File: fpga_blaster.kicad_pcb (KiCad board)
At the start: 2 copper layers, 193 x 81.9 mm, 238 parts, among them J1 Conn_02x05_Odd_Even, J2 Conn_02x05_Odd_Even, J3 Conn_01x03, J4 Conn_02x05_Odd_Even, J5 HDMI_D_1.4, J8 HDMI_D_1.4, Q1 Pmos, Q2 2N3904, Q4 IPD60R145, Q6 IPD60R145, Q7 2N3906, Q9 2N3904, SW1 FIRE, SW2 SW_DIP_x03, SW3 ARM, U1 LT3420, U10 AMC3330, U11 TLV9102, U12 LTC6362, U13 TLV9102, U14 AMC3302, U15 LTC6362, U16 LTC6362, U17 AD7352, U18 IR2127, U19 S80KS2563GABHV020, U2 MAX10, U20 TLV74318, U21 LM809, U22 MAX3227, U3 AD7352, U4 TLV74325, U5 4945, U6 4945, U7 LTC6362, U8 AMC3330, U9 AMC3302, X1 ASE-48MHz

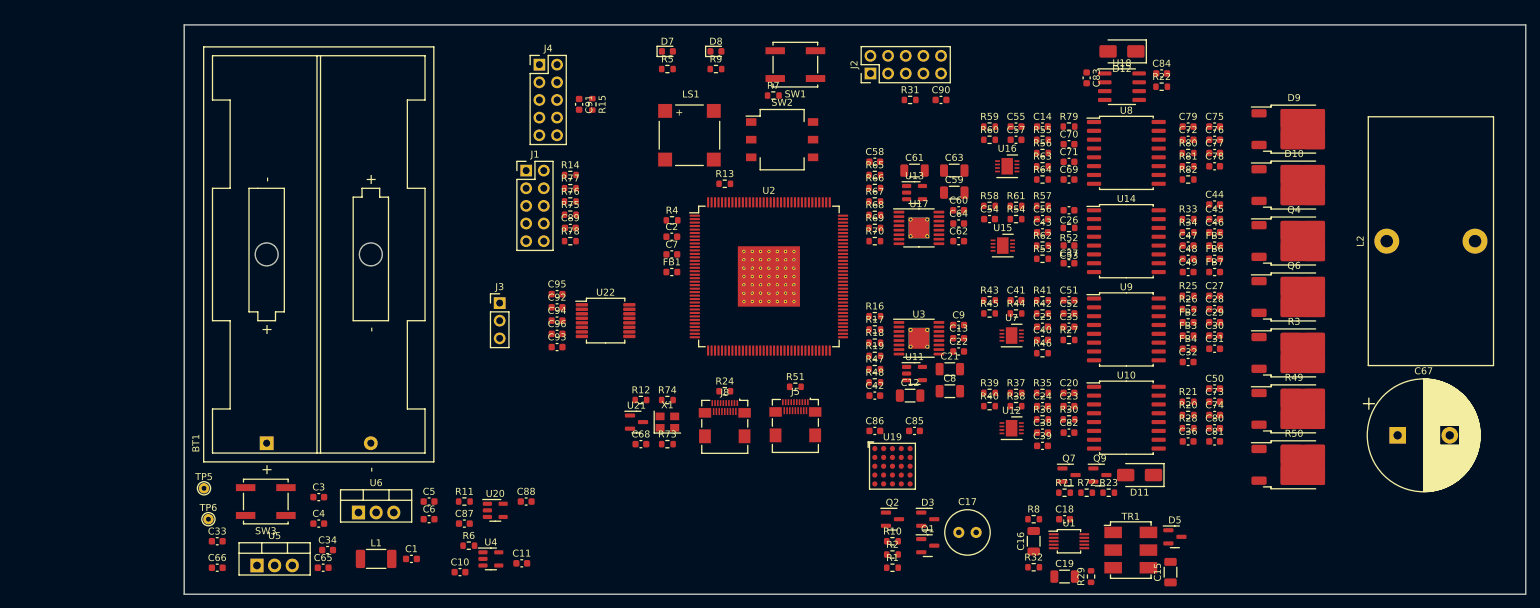
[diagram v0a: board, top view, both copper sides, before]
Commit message: PCB V0.8 tapeout
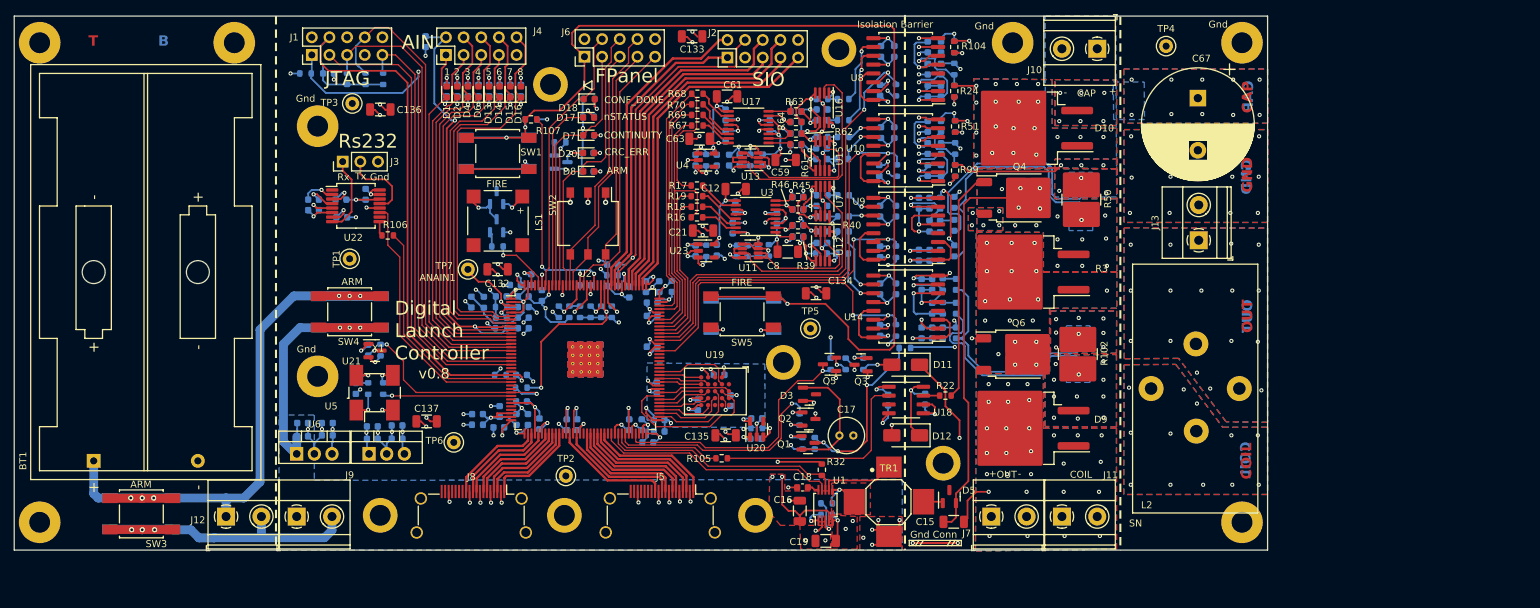
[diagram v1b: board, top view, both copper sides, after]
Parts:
- removed L1: 600uH 0.5A, Inductor_SMD:L_2010_5025Metric
- removed Q9: 2N3904, Package_TO_SOT_SMD:SOT-23
- added ?: , , F.Cu at (223.4, 97.3)
- added ?: , , F.Cu at (223.4, 109.9)
- added C100: 0.1u, Capacitor_SMD:C_0603_1608Metric, B.Cu at (146.1, 108.3)
- added C101: 0.1u, Capacitor_SMD:C_0603_1608Metric, B.Cu at (141.8, 89.9)
- added C102: 0.1u, Capacitor_SMD:C_0603_1608Metric, B.Cu at (134.3, 109.0)
- added C103: 0.1u, Capacitor_SMD:C_0603_1608Metric, B.Cu at (127.3, 108.2)
- added C104: 0.1u, Capacitor_SMD:C_0603_1608Metric, B.Cu at (123.1, 109.3)
- added C105: 0.1u, Capacitor_SMD:C_0603_1608Metric, B.Cu at (123.4, 90.5)
- added C106: 0.1u, Capacitor_SMD:C_0603_1608Metric, B.Cu at (146.1, 89.1)
- added C107: 0.1u, Capacitor_SMD:C_0603_1608Metric, B.Cu at (125.4, 88.9)
- added C108: 0.1u, Capacitor_SMD:C_0603_1608Metric, B.Cu at (126.6, 90.5)
- added C109: 0.1u, Capacitor_SMD:C_0603_1608Metric, B.Cu at (123.2, 107.1)
- added C110: 0.1u, Capacitor_SMD:C_0603_1608Metric, B.Cu at (143.6, 109.0)
- added C111: 0.1u, Capacitor_SMD:C_0603_1608Metric, B.Cu at (127.7, 88.1)
- added C112: 0.1u, Capacitor_SMD:C_0603_1608Metric, B.Cu at (145.1, 91.4)
- added C113: 0.1u, Capacitor_SMD:C_0603_1608Metric, B.Cu at (125.6, 108.2)
- added C114: 0.1u, Capacitor_SMD:C_0603_1608Metric, B.Cu at (126.6, 95.1)
- added C115: 0.1u, Capacitor_SMD:C_0603_1608Metric, B.Cu at (126.3, 101.8)
- added C116: 0.1u, Capacitor_SMD:C_0603_1608Metric, B.Cu at (126.3, 105.6)
- added C117: 0.1u, Capacitor_SMD:C_0603_1608Metric, B.Cu at (132.8, 109.0)
- added C118: 0.1u, Capacitor_SMD:C_0603_1608Metric, B.Cu at (141.8, 109.0)
- added C119: 0.1u, Capacitor_SMD:C_0603_1608Metric, B.Cu at (145.8, 103.6)
- added C120: 0.1u, Capacitor_SMD:C_0603_1608Metric, B.Cu at (139.4, 85.9)
- added C121: 0.1u, Capacitor_SMD:C_0603_1608Metric, B.Cu at (129.3, 90.4)
- added C122: 0.1u, Capacitor_SMD:C_0603_1608Metric, B.Cu at (135.5, 88.9)
- added C123: 0.1u, Capacitor_SMD:C_0603_1608Metric, B.Cu at (145.1, 93.3)
- added C124: 0.1u, Capacitor_SMD:C_0603_1608Metric, B.Cu at (145.1, 97.7)
- added C125: 0.1u, Capacitor_SMD:C_0603_1608Metric, B.Cu at (128.9, 108.8)
- added C126: 0.1u, Capacitor_SMD:C_0603_1608Metric, B.Cu at (156.2, 70.9)
- added C127: 0.1u, Capacitor_SMD:C_0603_1608Metric, B.Cu at (157.4, 84.0)
- added C128: 1u, Capacitor_SMD:C_0603_1608Metric, B.Cu at (151.4, 83.9)
- added C129: 1u, Capacitor_SMD:C_0603_1608Metric, B.Cu at (154.4, 83.8)
- added C130: 1u, Capacitor_SMD:C_0603_1608Metric, B.Cu at (120.0, 107.4)
- added C131: 0.1u, Capacitor_SMD:C_0603_1608Metric, B.Cu at (102.5, 103.7)
- added C132: 4.7u, Capacitor_SMD:C_1206_3216Metric, F.Cu at (122.9, 86.6)
- added C133: 4.7u, Capacitor_SMD:C_1206_3216Metric, F.Cu at (150.9, 53.1)
- added C134: 4.7u, Capacitor_SMD:C_1206_3216Metric, F.Cu at (168.7, 90.1)
- added C135: 4.7u, Capacitor_SMD:C_1206_3216Metric, F.Cu at (155.7, 110.5)
- added C136: 4.7u, Capacitor_SMD:C_1206_3216Metric, F.Cu at (106.0, 63.6)
- added C137: 4.7u, Capacitor_SMD:C_1206_3216Metric, F.Cu at (112.7, 108.5)
- added C97: 0.1u, Capacitor_SMD:C_0603_1608Metric, B.Cu at (154.7, 101.8)
- added C98: 0.1u, Capacitor_SMD:C_0603_1608Metric, B.Cu at (144.2, 89.1)
- added C99: 0.1u, Capacitor_SMD:C_0603_1608Metric, B.Cu at (146.1, 109.9)
- added D1: Yel, LED_SMD:LED_0603_1608Metric, F.Cu at (117.1, 61.1)
- added D13: Yel, LED_SMD:LED_0603_1608Metric, F.Cu at (121.7, 61.1)
- added D14: Yel, LED_SMD:LED_0603_1608Metric, F.Cu at (123.2, 61.1)
- added D15: Yel, LED_SMD:LED_0603_1608Metric, F.Cu at (124.7, 61.1)
- added D16: Yel, LED_SMD:LED_0603_1608Metric, F.Cu at (126.2, 61.1)
- added D17: nSTATUS, LED_SMD:LED_0603_1608Metric, F.Cu at (136.0, 64.8)
- added D18: CONF_DONE, LED_SMD:LED_0603_1608Metric, F.Cu at (136.1, 62.1)
- added D19: BAV99, Package_TO_SOT_SMD:SOT-23, B.Cu at (122.7, 76.3)
- added D2: Yel, LED_SMD:LED_0603_1608Metric, F.Cu at (115.6, 61.1)
- added D20: CRC_ERR, LED_SMD:LED_0603_1608Metric, F.Cu at (136.0, 69.8)
- added D4: Yel, LED_SMD:LED_0603_1608Metric, F.Cu at (118.6, 61.1)
- added D6: Yel, LED_SMD:LED_0603_1608Metric, F.Cu at (120.1, 61.1)
- added FB10: Ferrite, Inductor_SMD:L_0603_1608Metric, B.Cu at (120.0, 109.0)
- added FB11: Ferrite, Inductor_SMD:L_0603_1608Metric, B.Cu at (144.5, 111.5)
- added FB8: Ferrite, Inductor_SMD:L_0603_1608Metric, B.Cu at (148.0, 89.1)
- added FB9: Ferrite, Inductor_SMD:L_0603_1608Metric, B.Cu at (120.9, 91.3)
- added H1: ~, MountingHole:MountingHole_3mm_Pad, F.Cu at (57.0, 54.0)
- added H10: ~, MountingHole:MountingHole_3mm_Pad, F.Cu at (57.0, 123.0)
- added H11: ~, MountingHole:MountingHole_3mm_Pad, F.Cu at (130.5, 60.0)
- added H12: ~, MountingHole:MountingHole_3mm_Pad, F.Cu at (230.0, 123.0)
- added H13: ~, MountingHole:MountingHole_3mm_Pad, F.Cu at (160.0, 122.0)
- added H14: ~, MountingHole:MountingHole_3mm_Pad, F.Cu at (106.0, 122.0)
- added H15: ~, MountingHole:MountingHole_3mm_Pad, F.Cu at (187.0, 114.5)
- added H2: ~, MountingHole:MountingHole_3mm_Pad, F.Cu at (85.0, 54.0)
- added H3: ~, MountingHole:MountingHole_3mm_Pad, F.Cu at (172.0, 55.0)
- added H4: ~, MountingHole:MountingHole_3mm_Pad, F.Cu at (197.0, 54.0)
- added H5: ~, MountingHole:MountingHole_3mm_Pad, F.Cu at (230.0, 54.0)
- added H6: ~, MountingHole:MountingHole_3mm_Pad, F.Cu at (97.0, 66.0)
- added H7: ~, MountingHole:MountingHole_3mm_Pad, F.Cu at (97.0, 102.0)
- added H8: ~, MountingHole:MountingHole_3mm_Pad, F.Cu at (164.0, 100.0)
- added H9: ~, MountingHole:MountingHole_3mm_Pad, F.Cu at (132.5, 122.0)
- added J10: Screw_Terminal_01x02, TerminalBlock_Phoenix:TerminalBlock_Phoenix_MKDS-1,5-2-5.08_1x02_P5.08mm_Horizontal, F.Cu at (209.2, 54.9)
- added J11: Screw_Terminal_01x02, TerminalBlock_Phoenix:TerminalBlock_Phoenix_MKDS-1,5-2-5.08_1x02_P5.08mm_Horizontal, F.Cu at (204.1, 122.2)
- added J12: Screw_Terminal_01x02, TerminalBlock_Phoenix:TerminalBlock_Phoenix_MKDS-1,5-2-5.08_1x02_P5.08mm_Horizontal, F.Cu at (83.8, 122.2)
- added J13: Screw_Terminal_01x02, TerminalBlock_Phoenix:TerminalBlock_Phoenix_MKDS-1,5-2-5.08_1x02_P5.08mm_Horizontal, F.Cu at (223.8, 82.4)
- added J6: Conn_02x05_Odd_Even, Connector_PinHeader_2.54mm:PinHeader_2x05_P2.54mm_Vertical, F.Cu at (135.4, 56.0)
- added J7: Screw_Terminal_01x02, TerminalBlock_Phoenix:TerminalBlock_Phoenix_MKDS-1,5-2-5.08_1x02_P5.08mm_Horizontal, F.Cu at (193.9, 122.2)
- added J9: Screw_Terminal_01x02, TerminalBlock_Phoenix:TerminalBlock_Phoenix_MKDS-1,5-2-5.08_1x02_P5.08mm_Horizontal, F.Cu at (94.0, 122.2)
- added Q3: 2N3906, Package_TO_SOT_SMD:SOT-23, F.Cu at (175.2, 100.3)
- added Q5: 2N3904, Package_TO_SOT_SMD:SOT-23, F.Cu at (170.6, 100.3)
- added Q8: 2N3904, Package_TO_SOT_SMD:SOT-23, B.Cu at (132.0, 71.2)
- added R100: 0R, Resistor_SMD:R_0603_1608Metric, B.Cu at (206.9, 78.7)
- added R101: 0R, Resistor_SMD:R_0603_1608Metric, B.Cu at (206.9, 74.4)
- added R102: 0.005R 1W, myspace pcb:R_2818 current sense, F.Cu at (206.4, 98.8)
- added R103: 0R, Resistor_SMD:R_0603_1608Metric, B.Cu at (206.5, 96.8)
- added R104: 0R, Resistor_SMD:R_0603_1608Metric, F.Cu at (188.6, 54.6)
- added R105: 22R, Resistor_SMD:R_0603_1608Metric, F.Cu at (155.1, 113.8)
- added R106: 22R, Resistor_SMD:R_0603_1608Metric, F.Cu at (107.1, 81.7)
- added R107: 22R, Resistor_SMD:R_0603_1608Metric, F.Cu at (127.7, 65.0)
- added R108: 1K, Resistor_SMD:R_0603_1608Metric, B.Cu at (122.9, 83.3)
- added R109: 1K, Resistor_SMD:R_0603_1608Metric, B.Cu at (135.8, 69.8)
- added R110: 0R, Resistor_SMD:R_0603_1608Metric, B.Cu at (181.5, 97.9)
- added R111: 1K, Resistor_SMD:R_0603_1608Metric, B.Cu at (131.9, 68.3)
- added R112: DNI, Resistor_SMD:R_0603_1608Metric, B.Cu at (126.3, 103.6)
- added R83: 1K, Resistor_SMD:R_0603_1608Metric, B.Cu at (117.1, 60.8)
- added R84: 1K, Resistor_SMD:R_0603_1608Metric, B.Cu at (115.6, 60.8)
- added R85: 1K, Resistor_SMD:R_0603_1608Metric, B.Cu at (118.6, 60.8)
- added R86: 1K, Resistor_SMD:R_0603_1608Metric, B.Cu at (120.1, 60.8)
- added R87: 1K, Resistor_SMD:R_0603_1608Metric, B.Cu at (121.7, 60.8)
- added R88: 1K, Resistor_SMD:R_0603_1608Metric, B.Cu at (123.2, 60.8)
- added R89: 1K, Resistor_SMD:R_0603_1608Metric, B.Cu at (124.7, 60.8)
- added R90: 1K, Resistor_SMD:R_0603_1608Metric, B.Cu at (126.2, 60.8)
- added R91: 1K, Resistor_SMD:R_0603_1608Metric, B.Cu at (136.0, 64.6)
- added R92: 1K, Resistor_SMD:R_0603_1608Metric, B.Cu at (136.0, 62.1)
- added R93: DNI, Resistor_SMD:R_0603_1608Metric, B.Cu at (133.2, 92.7)
- added R94: DNI, Resistor_SMD:R_0603_1608Metric, B.Cu at (134.7, 92.7)
- added R95: 10K, Resistor_SMD:R_0603_1608Metric, B.Cu at (131.7, 92.7)
- added R96: DNI, Resistor_SMD:R_0603_1608Metric, B.Cu at (137.8, 92.7)
- added R97: DNI, Resistor_SMD:R_0603_1608Metric, B.Cu at (136.3, 92.7)
- added R98: 10K, Resistor_SMD:R_0603_1608Metric, B.Cu at (152.9, 83.9)
- added R99: 0R, Resistor_SMD:R_0603_1608Metric, F.Cu at (188.7, 72.4)
- added SW4: ARM, myspace pcb:SW_SPST_HP03, F.Cu at (101.6, 92.7)
- added SW5: FIRE, myspace pcb:SW_SPST_HP03, F.Cu at (158.1, 92.7)
- added SW6: FIRE, myspace pcb:SW_SPST_HP03, B.Cu at (158.1, 93.1)
- added SW7: ARM, myspace pcb:SW_SPST_HP03, B.Cu at (101.7, 92.7)
- added SW8: ARM, myspace pcb:SW_SPST_HP03, B.Cu at (71.6, 121.8)
- added SW9: FIRE, myspace pcb:SW_SPST_HP03, B.Cu at (122.9, 69.9)
- added TP1: ~, TestPoint:TestPoint_Keystone_5000-5004_Miniature, F.Cu at (101.6, 85.1)
- added TP2: ~, TestPoint:TestPoint_Keystone_5000-5004_Miniature, F.Cu at (132.7, 116.3)
- added TP3: ~, TestPoint:TestPoint_Keystone_5000-5004_Miniature, F.Cu at (102.0, 62.7)
- added TP4: ~, TestPoint:TestPoint_Keystone_5000-5004_Miniature, F.Cu at (219.1, 54.5)
- added TP7: ~, TestPoint:TestPoint_Keystone_5000-5004_Miniature, F.Cu at (118.6, 86.6)
- added U23: TLV74325, Package_TO_SOT_SMD:SOT-23-5, F.Cu at (152.9, 83.9)
- BT1: value 2xAA Li -> ~
- C1, C10, C11, C13, C14, C20, C22, C24, C25, C26, C3, C30, C33, C34, C4, C42, C43, C45, C5, C50, C51, C58, C6, C60, C62, C64, C65, C66, C68, C7, C70, C75, C83, C84, C87, C88, C89, C9, C90, C91, C92, C93, C94, C95, C96, FB1, FB2, FB3, FB4, FB5, FB6, FB7, R1, R10, R11, R13, R14, R15, R2, R20, R21, R23, R25, R26, R27, R28, R29, R30, R31, R33, R34, R35, R36, R37, R38, R4, R41, R42, R43, R44, R5, R52, R53, R54, R55, R56, R57, R58, R59, R6, R60, R7, R71, R72, R73, R75, R76, R77, R78, R79, R8, R80, R81, R82, R9: moved to B.Cu
- C17: footprint Capacitor_THT:C_Radial_D6.3mm_H5.0mm_P2.50mm -> Capacitor_THT:C_Radial_D5.0mm_H7.0mm_P2.00mm
- C2: value 0.1u -> 0.001u; moved to B.Cu
- C23, C28, C31, C37, C38, C39, C40, C41, C47, C48, C52, C54, C55, C56, C57, C71, C74, C77, C78, C80: value 1n -> 0.001u; moved to B.Cu
- C27, C36, C44, C72: value 10n -> 0.01u; moved to B.Cu
- C29, C32, C35, C46, C49, C53, C69, C73, C76, C79, C81, C82: value 100n -> 0.1u; moved to B.Cu
- C85: value 1u -> 0.1u; moved to B.Cu
- C86: value 1n -> 0.1u; moved to B.Cu
- D10, D9, R3: footprint Package_TO_SOT_SMD:TO-252-2 -> Package_TO_SOT_SMD:TO-263-2_TabPin1
- D11, D12: value SBYV26C -> ES1J
- D3: value 1N4001 -> BAV99
- D5: value MMBD3004SE -> GSD2004S
- D7: value FIRE -> CONTINUITY
- J5, J8: footprint Connector_HDMI:HDMI_Micro-D_Molex_46765-0x01 -> Connector_HDMI:HDMI_A_Amphenol_10029449-x01xLF_Horizontal
- Q1: value Pmos -> STR2P3LLH6(Pfet)
- Q7: value 2N3906 -> 2N3904; moved to B.Cu
- R12, R74: value 1K -> 22R; moved to B.Cu
- R22: value 2R -> 10R
- R39, R40, R45, R46, R61, R62, R63, R64: value 30R -> 22R
- R47, R48, R65, R66: value 10.0K -> 10.01K; moved to B.Cu
- R49: value 0.005R 1W -> 0R; footprint Package_TO_SOT_SMD:TO-252-2 -> Resistor_SMD:R_0603_1608Metric; moved to B.Cu
- R50: footprint Package_TO_SOT_SMD:TO-252-2 -> myspace pcb:R_2818 current sense
- SW1, SW3: footprint Button_Switch_SMD:SW_Push_1P1T_NO_CK_KSC6xxJ -> myspace pcb:SW_SPST_HP03
- TP5: value 3V -> ~; footprint TestPoint:TestPoint_THTPad_D1.5mm_Drill0.7mm -> TestPoint:TestPoint_Keystone_5000-5004_Miniature
- TP6: value GND -> ~; footprint TestPoint:TestPoint_THTPad_D1.5mm_Drill0.7mm -> TestPoint:TestPoint_Keystone_5000-5004_Miniature
- TR1: footprint RF_Mini-Circuits:Mini-Circuits_CD542_H2.84mm -> myspace pcb:PA0637A Pulse Coil
- U11, U13: value TLV9102 -> TLV9062xD; footprint Package_TO_SOT_SMD:SOT-23-5 -> Package_TO_SOT_SMD:SOT-23-8
- U12, U15, U16, U7: footprint Package_DFN_QFN:DFN-8-1EP_3x3mm_P0.5mm_EP1.66x2.38mm -> Package_SO:MSOP-8_3x3mm_P0.65mm
- U17, U3: footprint Package_SO:TSSOP-16-1EP_4.4x5mm_P0.65mm_EP3x3mm_ThermalVias -> Package_SO:TSSOP-16_4.4x5mm_P0.65mm
- U19: footprint Package_BGA:BGA-25_6.35x6.35mm_Layout5x5_P1.27mm -> myspace pcb:FBGA-24_6mmx8mm_Layout5x5_P1.00mm
- U2: value MAX10 -> MAX10M04; footprint Package_QFP:EQFP-144-1EP_20x20mm_P0.5mm_EP8.93x8.7mm_ThermalVias -> Package_QFP:EQFP-144-1EP_20x20mm_P0.5mm_EP5x5mm_ThermalVias
- U5: value 4945 -> LMO78_03-1.0
- X1: footprint Oscillator:Oscillator_SMD_Abracon_ASE-4Pin_3.2x2.5mm -> Oscillator:Oscillator_SMD_Abracon_ASV-4Pin_7.0x5.1mm_HandSoldering
- moved TP5 90.2 mm to (167.9, 95.1)
- moved Q7 89.8 mm to (122.7, 80.3), turned to 90 degrees
- moved C10 68.3 mm to (151.4, 70.9), turned to -90 degrees
- moved U4 65.2 mm to (152.9, 70.9)
- moved R6 65.1 mm to (152.9, 70.9), turned to -90 degrees
- moved C11 64.4 mm to (154.4, 70.9), turned to -90 degrees
- moved D12 63.4 mm to (181.6, 110.5)
- moved C81 59.0 mm to (184.8, 69.2), turned to -90 degrees
- moved C74 58.5 mm to (184.8, 66.0), turned to -90 degrees
- moved D9 58.3 mm to (198.1, 109.5), turned to 180 degrees
- moved C84 57.9 mm to (184.4, 105.3), turned to -90 degrees
- moved C36 57.6 mm to (186.7, 66.0), turned to 90 degrees
- moved C67 56.4 mm to (223.6, 62.0), turned to -90 degrees
- moved C80 55.5 mm to (184.8, 72.4), turned to 90 degrees
- moved U18 54.7 mm to (181.7, 105.4)
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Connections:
- net Net-(BT1-+) renamed /B+
- net Net-(J1-Pin_4) renamed /VCCIO1B
- net Net-(J4-Pin_2) renamed /VCCIO1A
- net Net-(Q6-D) renamed /SWDIS
- net Net-(U1-SW) renamed /SW
- net Net-(U10-DCDC_HGND) renamed /HGNDCV
- net Net-(U14-DCDC_HGND) renamed /HGNDLI
- net Net-(U2A-ANAIN1) renamed /ANAIN1
- net Net-(U8-DCDC_HGND) renamed /HGNDLV
- net Net-(U8-OUTN) renamed /LVoutn
- net Net-(U8-OUTP) renamed /LVoutp
- net Net-(U9-DCDC_HGND) renamed /HGNDCI
- net Net-(U9-OUTN) renamed /CIoutn
- net Net-(U9-OUTP) renamed /CIoutp
- BT1 pad 2: CVlo -> GND
- C1 pad 2: CVlo -> GND
- C10 pad 2: CVlo -> GND
- C11 pad 2: CVlo -> GND
- C12 pad 2: CVlo -> GND
- C13 pad 2: CVlo -> GND
- C14 pad 1: +2V5 -> +3.3V
- C14 pad 2: CVlo -> GND
- C15 pad 1: CIlo -> +300V
- C15 pad 2: CVlo -> GND
- C16 pad 2: CVlo -> GND
- C17 pad 2: CVlo -> GND
- C18 pad 2: CVlo -> GND
- C19 pad 2: CVlo -> GND
- C2 pad 2: CVlo -> /REFGND
- C20 pad 2: CVlo -> GND
- C21 pad 2: CVlo -> GND
- C22 pad 2: CVlo -> GND
- C23 pad 2: CVlo -> GND
- C24 pad 1: +2V5 -> +3.3V
- C24 pad 2: CVlo -> GND
- C25 pad 1: +2V5 -> +3.3V
- C25 pad 2: CVlo -> GND
- C26 pad 2: CVlo -> GND
- C3 pad 2: CVlo -> GND
- C33 pad 2: CVlo -> GND
- C34 pad 2: CVlo -> GND
- C37 pad 2: CVlo -> GND
- C38 pad 1: /vinb0+ -> /vina0+
- C38 pad 2: CVlo -> GND
- C39 pad 1: /vinb0- -> /vina0-
- C39 pad 2: CVlo -> GND
- C4 pad 2: CVlo -> GND
- C40 pad 1: /vina0+ -> /vinb0+
- C40 pad 2: CVlo -> GND
- C41 pad 1: /vina0- -> /vinb0-
- C41 pad 2: CVlo -> GND
- C42 pad 2: CVlo -> GND
- C43 pad 1: +2V5 -> +3.3V
- C43 pad 2: CVlo -> GND
- C5 pad 2: CVlo -> GND
- C51 pad 2: CVlo -> GND
- C52 pad 2: CVlo -> GND
- C54 pad 2: CVlo -> GND
- C55 pad 2: CVlo -> GND
- C56 pad 2: CVlo -> GND
- C57 pad 2: CVlo -> GND
- C58 pad 2: CVlo -> GND
- C59 pad 2: CVlo -> GND
- C6 pad 2: CVlo -> GND
- C60 pad 2: CVlo -> GND
- C61 pad 2: CVlo -> GND
- C62 pad 2: CVlo -> GND
- C63 pad 2: CVlo -> GND
- C64 pad 2: CVlo -> GND
- C65 pad 2: CVlo -> GND
- C66 pad 2: CVlo -> GND
- C67 pad 1: CIhi -> /CSEN
- C67 pad 2: CVlo -> GND
- C68 pad 2: CVlo -> GND
- C7 pad 2: CVlo -> GND
- C70 pad 2: CVlo -> GND
- C71 pad 2: CVlo -> GND
- C8 pad 2: CVlo -> GND
- C83 pad 2: CVlo -> GND
- C84 pad 2: Net-(D9-K) -> +VSW
- C85 pad 2: CVlo -> GND
- C86 pad 2: CVlo -> GND
- C87 pad 2: CVlo -> GND
- C88 pad 2: CVlo -> GND
- C89 pad 2: CVlo -> GND
- C9 pad 2: CVlo -> GND
- C90 pad 1: Net-(J2-Pin_10) -> /vccio7
- C90 pad 2: CVlo -> GND
- C91 pad 2: CVlo -> GND
- C93 pad 2: CVlo -> GND
- C95 pad 2: CVlo -> GND
- C96 pad 2: CVlo -> GND
- D10 pad 1: LIhi -> /+OUT
- D10 pad 2: CIlo -> +300V
- D11 pad 1: IGNITER+ -> /+OUT
- D5 pad 2: CIlo -> +300V
- D9 pad 1: CVlo -> GND
- D9 pad 2: Net-(D9-K) -> +VSW
- FB1 pad 1: Net-(U2A-REFGDN) -> /REFGND
- FB1 pad 2: CVlo -> GND
- FB6 pad 2: IGNITER+ -> LIlo
- FB7 pad 2: IGNITER+ -> LIlo
- J1 pad 10: CVlo -> GND
- J1 pad 2: CVlo -> GND
- J2 pad 1: Net-(J2-Pin_1) -> /dio0
- J2 pad 10: Net-(J2-Pin_10) -> GND
- J2 pad 2: Net-(J2-Pin_2) -> /dio1
- J2 pad 3: Net-(J2-Pin_3) -> GND
- J2 pad 4: CVlo -> /vccio7
- J2 pad 5: CVlo -> /dio2
- J2 pad 6: Net-(J2-Pin_6) -> /dio3
- J2 pad 7: Net-(J2-Pin_7) -> /dio4
- J2 pad 8: Net-(J2-Pin_8) -> /dio5
- J2 pad 9: Net-(J2-Pin_9) -> /dio6
- J3 pad 1: /tx232 -> /rx232
- J3 pad 2: /rx232 -> /tx232
- J3 pad 3: CVlo -> GND
- J4 pad 4: /ain_5 -> /ain_3
- J4 pad 5: /ain_3 -> /ain_4
- J4 pad 6: /ain_6 -> /ain_5
- J4 pad 7: /ain_4 -> /ain_6
- J4 pad 9: CVlo -> GND
- J5 pad 1: unconnected-(J5-HPD/HEAC--Pad1) -> /hdmi2_d2+
- J5 pad 10: unconnected-(J5-D0S-Pad10) -> /hdmi2_ck+
- J5 pad 11: /hdmi_d0- -> GND
- J5 pad 12: /hdmi_ck+ -> /hdmi2_ck-
- J5 pad 14: /hdmi_ck- -> unconnected-(J5-UTILITY-Pad14)
- J5 pad 16: CVlo -> unconnected-(J5-SDA-Pad16)
- J5 pad 17: unconnected-(J5-SCL-Pad17) -> GND
- J5 pad 2: unconnected-(J5-UTILITY/HEAC+-Pad2) -> GND
- J5 pad 3: /hdmi_d2+ -> /hdmi2_d2-
- J5 pad 4: unconnected-(J5-D2S-Pad4) -> /hdmi2_d1+
- J5 pad 5: /hdmi_d2- -> GND
- J5 pad 6: /hdmi_d1+ -> /hdmi2_d1-
- J5 pad 7: unconnected-(J5-D1S-Pad7) -> /hdmi2_d0+
- J5 pad 8: /hdmi_d1- -> GND
- J5 pad 9: /hdmi_d0+ -> /hdmi2_d0-
- J5 pad SH: Net-(J5-PadSH) -> GND
- J8 pad 1: unconnected-(J8-HPD/HEAC--Pad1) -> /hdmi_d2+
- J8 pad 10: unconnected-(J8-D0S-Pad10) -> /hdmi_ck+
- J8 pad 11: /hdmi_d0- -> GND
- J8 pad 12: /hdmi_ck+ -> /hdmi_ck-
- J8 pad 14: /hdmi_ck- -> unconnected-(J8-UTILITY-Pad14)
- J8 pad 16: CVlo -> unconnected-(J8-SDA-Pad16)
- J8 pad 17: unconnected-(J8-SCL-Pad17) -> GND
- J8 pad 2: unconnected-(J8-UTILITY/HEAC+-Pad2) -> GND
- J8 pad 3: /hdmi_d2+ -> /hdmi_d2-
- J8 pad 4: unconnected-(J8-D2S-Pad4) -> /hdmi_d1+
- J8 pad 5: /hdmi_d2- -> GND
- J8 pad 6: /hdmi_d1+ -> /hdmi_d1-
- J8 pad 7: unconnected-(J8-D1S-Pad7) -> /hdmi_d0+
- J8 pad 8: /hdmi_d1- -> GND
- J8 pad 9: /hdmi_d0+ -> /hdmi_d0-
- J8 pad SH: Net-(J8-PadSH) -> GND
- L2 pad 1: Net-(D9-K) -> /LSEN
- L2 pad 2: LIhi -> /+OUT
- LS1 pad 1: /spk+ -> +3.3V
- LS1 pad 2: /spk- -> Net-(D19-A)
- Q2 pad 1: CVlo -> GND
- Q4 pad 1: Net-(Q4-G) -> /gate
- Q4 pad 2: CIlo -> +300V
- Q4 pad 3: Net-(D9-K) -> +VSW
- Q6 pad 1: Net-(Q1-D) -> /DisG
- Q6 pad 3: CVlo -> GND
- Q7 pad 1: +12V -> GND
- Q7 pad 3: Net-(Q7-C) -> Net-(D19-A)
- R1 pad 1: CVlo -> GND
- R18 pad 1: /dataa0 -> /dataA0
- R19 pad 1: /datab0 -> /dataB0
- R2 pad 1: CVlo -> GND
- R20 pad 1: CIhi -> CVhi
- R22 pad 1: /gate -> Net-(U18-HO)
- R22 pad 2: Net-(Q4-G) -> /gate
- R23 pad 1: Net-(Q7-B) -> Net-(Q3-B)
- R24 pad 1: Net-(J8-PadSH) -> LVhi
- R24 pad 2: CVlo -> /+OUT
- R3 pad 2: CIlo -> +300V
- R31 pad 2: Net-(J2-Pin_10) -> /vccio7
- R35 pad 1: Net-(U10-OUTN) -> /LIoutn
- R36 pad 1: Net-(U10-OUTP) -> /LIoutp
- R39 pad 2: /vinb0+ -> /vina0+
- R4 pad 2: CVlo -> GND
- R40 pad 2: /vinb0- -> /vina0-
- R45 pad 2: /vina0+ -> /vinb0+
- R46 pad 2: /vina0- -> /vinb0-
- R48 pad 1: CVlo -> GND
- R49 pad 1: IGNITER+ -> +VSW
- R50 pad 1: CIhi -> /CSEN
- R50 pad 2: CIlo -> +300V
- R51 pad 1: Net-(J5-PadSH) -> CVlo
- R51 pad 2: CVlo -> GND
- R53 pad 1: Net-(U14-OUTP) -> /CVoutp
- R54 pad 1: Net-(U14-OUTN) -> /CVoutn
- R66 pad 1: CVlo -> GND
- R69 pad 1: /dataa1 -> /dataA1
- R7 pad 2: CVlo -> GND
- R70 pad 1: /datab1 -> /dataB1
- R71 pad 2: Net-(Q7-C) -> Net-(Q3-C)
- R77 pad 2: /tdi -> /tms
- R78 pad 2: CVlo -> GND
- R8 pad 2: CVlo -> GND
- R80 pad 1: IGNITER+ -> LVhi
- R81 pad 1: CVlo -> LVlo
- SW2 pad 1: CVlo -> GND
- SW2 pad 2: CVlo -> GND
- SW2 pad 3: CVlo -> GND
- TP5 pad 1: +BATT -> GND
- TP6 pad 1: CVlo -> GND
- U1 pad 5: CVlo -> GND
- U10 pad 10: Net-(U10-OUTN) -> /CVoutn
- U10 pad 11: Net-(U10-OUTP) -> /CVoutp
- U10 pad 9: CVlo -> GND
- U11 pad 4: (no net) -> GND
- U11 pad 5: (no net) -> Net-(U11A-+)
- U12 pad 3: +2V5 -> +3.3V
- U12 pad 6: CVlo -> GND
- U12 pad 7: +2V5 -> +3.3V
- U13 pad 4: (no net) -> GND
- U13 pad 5: (no net) -> Net-(U13A-+)
- U14 pad 10: Net-(U14-OUTN) -> /LIoutn
- U14 pad 11: Net-(U14-OUTP) -> /LIoutp
- U14 pad 9: CVlo -> GND
- U15 pad 3: +2V5 -> +3.3V
- U15 pad 6: CVlo -> GND
- U15 pad 7: +2V5 -> +3.3V
- U16 pad 2: Net-(U13A--) -> Net-(U13B--)
- U16 pad 3: +2V5 -> +3.3V
- U16 pad 6: CVlo -> GND
- U16 pad 7: +2V5 -> +3.3V
- U17 pad 11: CVlo -> GND
- U17 pad 12: CVlo -> GND
- U17 pad 4: CVlo -> GND
- U17 pad 5: CVlo -> GND
- U18 pad 2: /pwm -> /pwmr
- U18 pad 4: CVlo -> GND
- U18 pad 5: Net-(D9-K) -> +VSW
- U18 pad 6: Net-(D9-K) -> +VSW
- U18 pad 7: /gate -> Net-(U18-HO)
- U19 pad A4: (no net) -> /spi_nrst
- U19 pad B1: unconnected-(U19-nCK-PadB1) -> +1V8
- U19 pad B3: CVlo -> GND
- U19 pad C1: CVlo -> GND
- U19 pad E5: CVlo -> GND
- U2 pad 10: /ain_4 -> /ain_5
- U2 pad 100: unconnected-(U2H-IO-Pad100) -> /dataB0
- U2 pad 101: /LIdiag -> /sclk
- U2 pad 102: /LVdiag -> /dataA1
- U2 pad 104: CVlo -> GND
- U2 pad 105: /CIdiag -> /dataB1
- U2 pad 106: /CVdiag -> /cs
- U2 pad 11: /ain_5 -> /ain_4
- U2 pad 110: Net-(J2-Pin_1) -> /dio6
- U2 pad 111: Net-(J2-Pin_3) -> /dio4
- U2 pad 112: Net-(J2-Pin_9) -> /dio5
- U2 pad 113: Net-(J2-Pin_7) -> /dio2
- U2 pad 114: Net-(J2-Pin_2) -> /dio3
- U2 pad 116: CVlo -> GND
- U2 pad 117: Net-(J2-Pin_10) -> /vccio7
- U2 pad 118: Net-(J2-Pin_6) -> /dio0
- U2 pad 119: Net-(J2-Pin_8) -> /dio1
- U2 pad 12: /ain_6 -> /ain_3
- U2 pad 121: unconnected-(U2J-DEVCLRN-Pad121) -> /devclrn
- U2 pad 122: unconnected-(U2J-DEVOE-Pad122) -> /devoe
- U2 pad 124: /fire -> Net-(R107-Pad1)
- U2 pad 125: CVlo -> GND
- U2 pad 126: unconnected-(U2J-BOOTSEL-Pad126) -> /bootsel
- U2 pad 129: unconnected-(U2J-NCONFIG-Pad129) -> Net-(U2J-NCONFIG)
- U2 pad 13: /ain_7 -> /ain_2
- U2 pad 133: CVlo -> GND
- U2 pad 134: unconnected-(U2J-CRC_ERR-Pad134) -> /crc
- U2 pad 136: unconnected-(U2J-NSTATUS-Pad136) -> /nstatus
- U2 pad 137: CVlo -> GND
- U2 pad 138: unconnected-(U2J-CONF_DONE-Pad138) -> /conf_done
- U2 pad 14: /ain_8 -> /ain_1
- U2 pad 142: CVlo -> GND
- U2 pad 145: CVlo -> GND
- U2 pad 21: /rx -> unconnected-(U2C-IO-Pad21)
- U2 pad 22: /tx -> unconnected-(U2C-IO-Pad22)
- U2 pad 24: unconnected-(U2C-IO-Pad24) -> /rx
- U2 pad 25: unconnected-(U2C-IO-Pad25) -> /tx
- U2 pad 38: /hdmi_d0- -> /hdmi_ck-
- U2 pad 39: /hdmi_d0+ -> /hdmi_ck+
- U2 pad 4: Net-(U2A-REFGDN) -> /REFGND
- U2 pad 41: /hdmi_d1- -> /hdmi_d0-
- U2 pad 42: CVlo -> GND
- U2 pad 43: /hdmi_d1+ -> /hdmi_d0+
- U2 pad 44: /hdmi_d2- -> /hdmi_d1-
- U2 pad 45: /hdmi_d2+ -> /hdmi_d1+
- U2 pad 46: /hdmi_ck- -> /hdmi_d2-
- U2 pad 47: /hdmi_ck+ -> /hdmi_d2+
- U2 pad 50: /hdmi_d0- -> /hdmi2_ck-
- U2 pad 52: /hdmi_d0+ -> /hdmi2_ck+
- U2 pad 53: CVlo -> GND
- U2 pad 55: /hdmi_d1- -> /hdmi2_d0-
- U2 pad 56: /hdmi_d1+ -> /hdmi2_d0+
- U2 pad 57: /hdmi_d2- -> /hdmi2_d1-
- U2 pad 58: /hdmi_d2+ -> /hdmi2_d1+
- U2 pad 59: /hdmi_ck- -> /hdmi2_d2-
- U2 pad 6: /ain_1 -> /ain_8
- U2 pad 60: /hdmi_ck+ -> /hdmi2_d2+
- U2 pad 62: unconnected-(U2F-IO-Pad62) -> /charge
- U2 pad 63: CVlo -> GND
- U2 pad 64: /dump -> /done
- U2 pad 66: /cont_n -> /dump
- U2 pad 68: CVlo -> GND
- U2 pad 69: /charge -> /cont_n
- U2 pad 7: /ain_2 -> /ain_7
- U2 pad 70: /done -> unconnected-(U2F-IO-Pad70)
- U2 pad 74: /spi_d1 -> /spi_ds
- U2 pad 75: /spi_d0 -> /spi_d2
- U2 pad 76: /spi_d6 -> /spi_d4
- U2 pad 77: /spi_d7 -> /spi_d3
- U2 pad 78: /spi_cs -> /spi_d0
- U2 pad 79: /spi_d2 -> /spi_d5
- U2 pad 8: /ain_3 -> /ain_6
- U2 pad 80: unconnected-(U2G-VREFB5N-Pad80) -> /spi_nrst
- U2 pad 81: /spi_d3 -> /spi_cs
- U2 pad 83: CVlo -> GND
- U2 pad 84: /spi_d5 -> /spi_d6
- U2 pad 85: /spi_clk -> /spi_d1
- U2 pad 86: /spi_d4 -> /spi_d7
- U2 pad 87: /spi_ds -> /spi_clk
- U2 pad 88: /dataB0 -> unconnected-(U2H-IO-Pad88)
- U2 pad 89: /dataB1 -> unconnected-(U2H-IO-Pad89)
- U2 pad 90: /dataA1 -> unconnected-(U2H-IO-Pad90)
- U2 pad 91: /dataA0 -> unconnected-(U2H-IO-Pad91)
- U2 pad 92: /cs -> unconnected-(U2H-IO-Pad92)
- U2 pad 93: /sclk -> /LIdiag
- U2 pad 95: CVlo -> GND
- U2 pad 96: unconnected-(U2H-IO-Pad96) -> /CIdiag
- U2 pad 97: unconnected-(U2H-VREFB6N-Pad97) -> /CVdiag
- U2 pad 98: unconnected-(U2H-IO-Pad98) -> /LVdiag
- U2 pad 99: unconnected-(U2H-IO-Pad99) -> /dataA0
- U20 pad 2: CVlo -> GND
- U21 pad 1: CVlo -> GND
- U22 pad 14: CVlo -> GND
- U22 pad 9: /rx -> Net-(U22-R1OUT)
- U3 pad 11: CVlo -> GND
- U3 pad 12: CVlo -> GND
- U3 pad 4: CVlo -> GND
- U3 pad 5: CVlo -> GND
- U4 pad 2: CVlo -> GND
- U5 pad 2: CVlo -> GND
- U6 pad 2: CVlo -> GND
- U7 pad 2: Net-(U11A--) -> Net-(U11B--)
- U7 pad 3: +2V5 -> +3.3V
- U7 pad 6: CVlo -> GND
- U7 pad 7: +2V5 -> +3.3V
- U8 pad 9: CVlo -> GND
- U9 pad 9: CVlo -> GND
- X1 pad 2: CVlo -> GND
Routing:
- net GND: track 0.00 -> 306.0 mm, vias 0 -> 154
- net +3.3V: track 0.00 -> 265.0 mm, vias 0 -> 74
- net /fire: track 0.00 -> 172.2 mm, vias 0 -> 3
- net +BATT: track 0.00 -> 106.6 mm, vias 0 -> 14
- net /B+: track 0.00 -> 96.0 mm, vias 0 -> 6
- net /VCCIO1B: track 0.00 -> 91.8 mm, vias 0 -> 1
- net /tck: track 0.00 -> 73.2 mm, vias 0 -> 1
- net /LVdiag: track 0.00 -> 69.2 mm, vias 0 -> 2
- net /jtagen: track 0.00 -> 68.8 mm
- net /tms: track 0.00 -> 66.6 mm
- net /tdo: track 0.00 -> 65.8 mm
- net /VCCIO1A: track 0.00 -> 62.2 mm, vias 0 -> 2
- net /CVdiag: track 0.00 -> 61.1 mm, vias 0 -> 2
- net /tdi: track 0.00 -> 60.7 mm
- net +300V: track 0.00 -> 58.0 mm, vias 0 -> 22
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- added copper zone on In2.Cu, net +12V
- added copper zone on B.Cu, net +1V8
- added copper zone on F.Cu, net +3.3V
- added copper zone on In2.Cu, net +3.3V
- added copper zone on B.Cu, net +300V
- added copper zone on F.Cu, net +300V
- added copper zone on In2.Cu, net +300V
- added copper zone on B.Cu, net +BATT
- added copper zone on F.Cu, net +BATT
- added copper zone on B.Cu, net +VSW
- added copper zone on F.Cu, net +VSW
- added copper zone on In1.Cu, net +VSW
- added copper zone on B.Cu, net /+OUT
- added copper zone on F.Cu, net /+OUT
- added copper zone on In1.Cu, net /+OUT
- added copper zone on B.Cu, net /CSEN
- added copper zone on F.Cu, net /CSEN
- added copper zone on In1.Cu, net /HGNDCI
- added copper zone on In1.Cu, net /HGNDCV
- added copper zone on In1.Cu, net /HGNDLI
- added copper zone on In1.Cu, net /HGNDLV
- added copper zone on B.Cu, net /LSEN
- added copper zone on F.Cu, net /LSEN
- added copper zone on In2.Cu, net /LSEN
- added copper zone on F.Cu, net /SW
- added copper zone on B.Cu, net /SWDIS
- added copper zone on F.Cu, net /SWDIS
- added copper zone on B.Cu, net GND
- added copper zone on F.Cu, net GND
- added copper zone on In1.Cu, net GND
- added copper zone on In2.Cu, net GND
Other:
- board size 193 x 81.9 mm -> 180.3 x 76.8 mm
- copper layers 2 -> 4
- board text added: "+"
- board text added: "-"
- board text added: "1"
- board text added: "2"
- board text added: "3"
- board text added: "4"
- board text added: "5"
- board text added: "6"
- board text added: "7"
- board text added: "8"
- board text added: "AIN"
- board text added: "ANAIN1"
- board text added: "ARM"
- board text added: "B"
- board text added: "CAP"
- board text added: "COIL"
- board text added: "CONF_DONE"
- board text added: "CONTINUITY"
- board text added: "CRC_ERR"
- board text added: "Digital Launch Controller"
- board text added: "DisG"
- board text added: "FPanel"
- board text added: "GND"
- board text added: "Gnd"
- board text added: "Gnd Conn"
- board text added: "Isolation Barrier"
- board text added: "JTAG"
- board text added: "OUT"
- board text added: "Rs232"
- board text added: "Rx"
- board text added: "SIO"
- board text added: "SN"
- board text added: "T"
- board text added: "Tx"
- board text added: "nSTATUS"
- board text added: "v0.8"
